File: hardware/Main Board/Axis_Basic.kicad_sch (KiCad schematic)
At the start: 57 parts, among them J1 USB_C_Receptacle_USB2.0, J2 JST_PH, J3 JST_PH, J4 S2B-PH-K-S, J5 1175-1628-ND, J6 1-84952-4, SW1 RKB2SJK, SW2 RKB2SJK, U1 TLV493D, U2 UA78M33CDCYR, U3 ATSAMD51J19A-AUT, U4 TMC2209-LA, U5 AT25040B-MAHL-T, Y1 SG-210STF 48.0000ML0

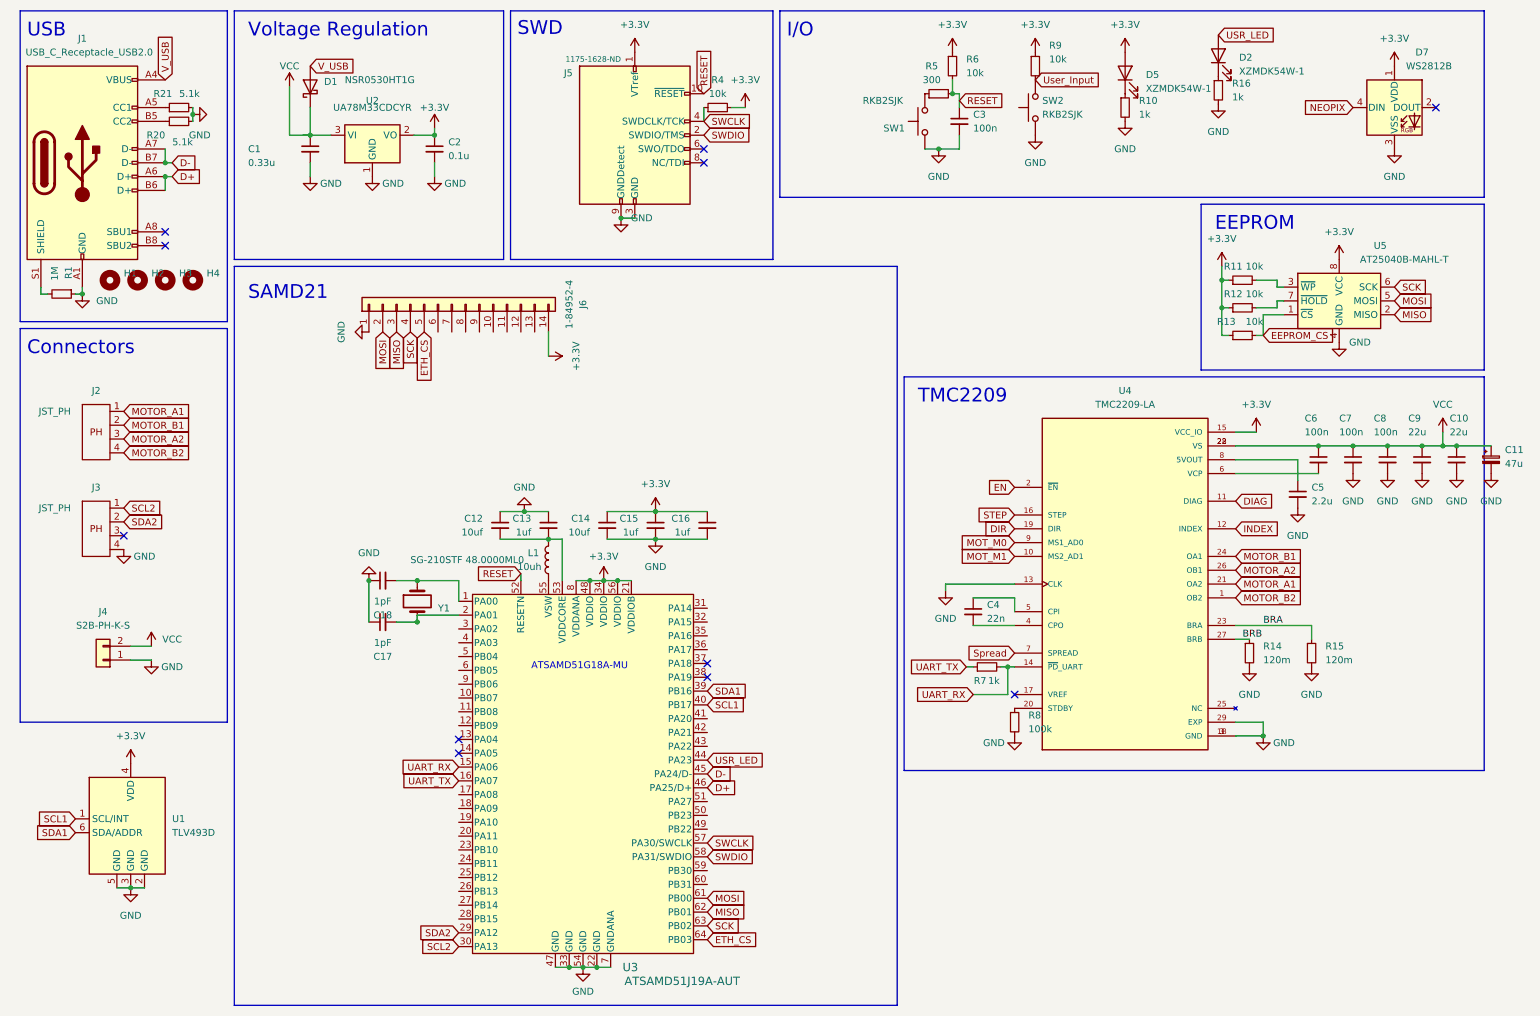
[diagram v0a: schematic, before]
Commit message: PCB V2 draft
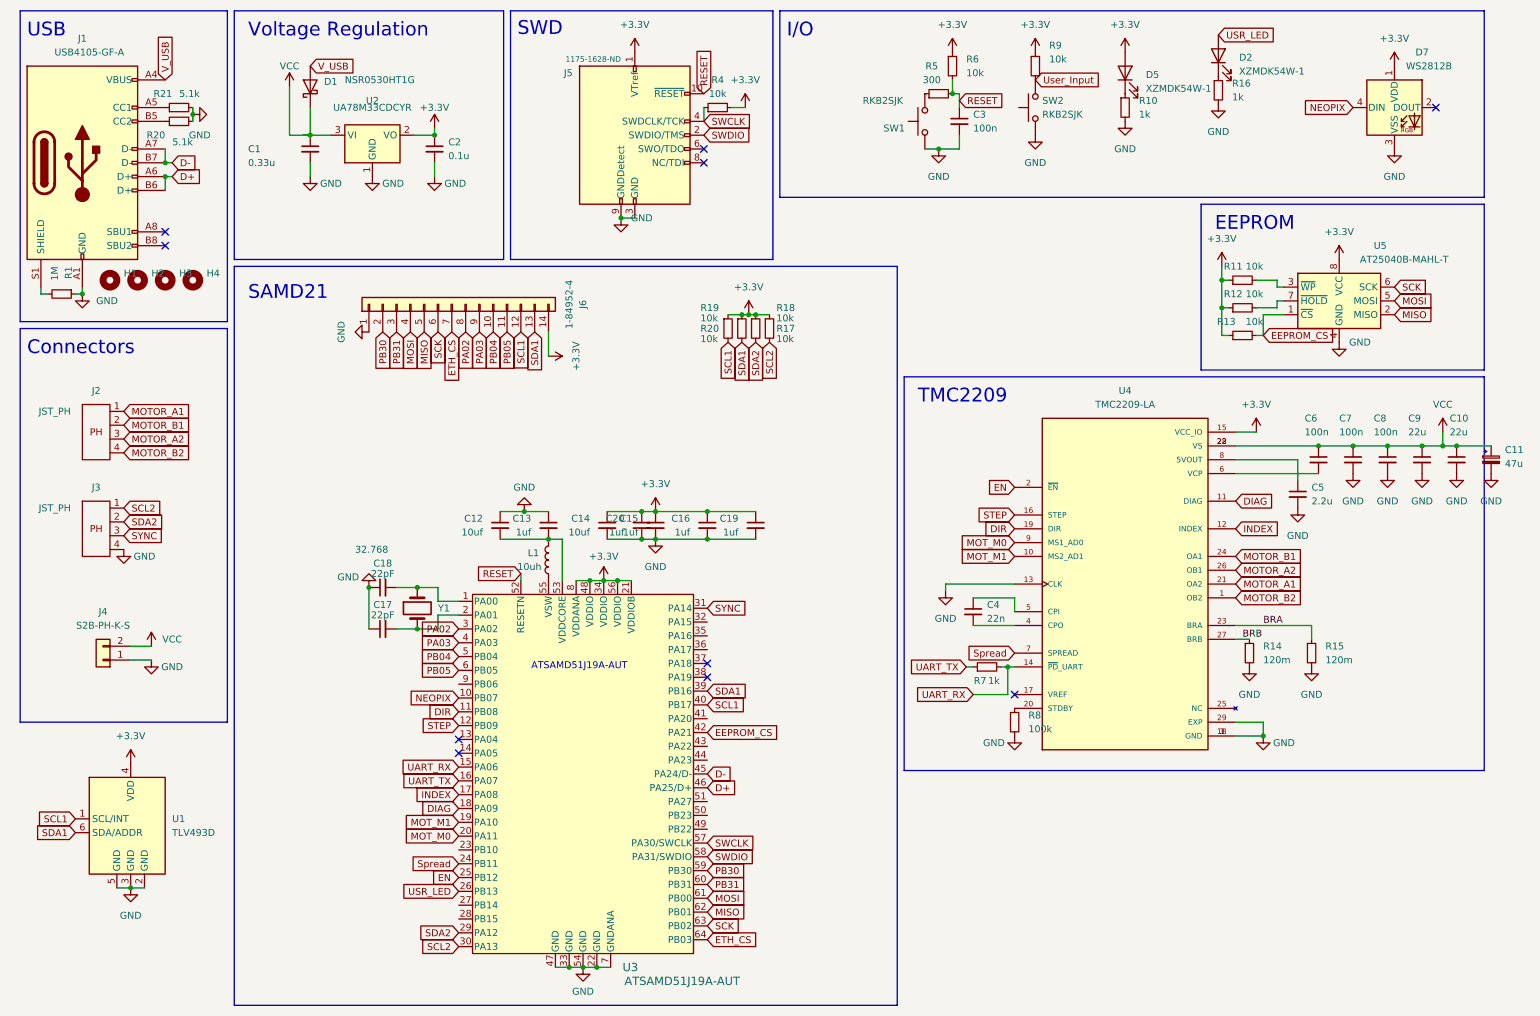
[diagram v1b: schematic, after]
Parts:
- added C19, C20: 1uf, Capacitor_SMD:C_0402_1005Metric, symbol Device:C_Small
- added R17, R18, R19, R20: 10k, Resistor_SMD:R_0402_1005Metric, symbol Device:R_Small
- C17, C18: value 1pF -> 22pF
- J1: value USB_C_Receptacle_USB2.0 -> USB4105-GF-A; footprint Connector_USB:USB_C_Receptacle_G-Switch_GT-USB-7010ASV -> Connector_USB:USB_C_Receptacle_GCT_USB4105-xx-A_16P_TopMnt_Horizontal
- Y1: value SG-210STF 48.0000ML0 -> 32.768; footprint Crystal:Crystal_SMD_2520-4Pin_2.5x2.0mm -> Crystal:Crystal_SMD_3215-2Pin_3.2x1.5mm
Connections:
- net +3.3V: now also C19.1, C20.1, R17.1, R18.1, R19.1, R20.1
- net DIAG: now also U3.18 (PA09)
- net DIR: now also U3.11 (PB08)
- net EEPROM_CS: now also U3.42 (PA21)
- net EN: now also U3.25 (PB12)
- net ETH_CS: now also J6.7 (Pin_7); no longer J6.5 (Pin_5)
- net GND: now also C19.2, C20.2
- net INDEX: now also U3.17 (PA08)
- net MISO: now also J6.5 (Pin_5); no longer J6.3 (Pin_3)
- net MOSI: now also J6.4 (Pin_4); no longer J6.2 (Pin_2)
- net MOT_M0: now also U3.20 (PA11)
- net MOT_M1: now also U3.19 (PA10)
- net NEOPIX: now also U3.10 (PB07)
- net SCK: now also J6.6 (Pin_6); no longer J6.4 (Pin_4)
- net SCL1: now also J6.12 (Pin_12), R20.2
- net SCL2: now also R17.2
- net SDA1: now also J6.13 (Pin_13), R19.2
- net SDA2: now also R18.2
- net STEP: now also U3.12 (PB09)
- net Spread: now also U3.24 (PB11)
- net USR_LED: now also U3.26 (PB13); no longer U3.44 (PA23)
- net PB04: now reaches J6.10 (Pin_10)
- net PB04: now also U3.5 (PB04)
- net PB05: now reaches J6.11 (Pin_11)
- net PB05: now also U3.6 (PB05)
- net PA02: now reaches J6.8 (Pin_8)
- net PA02: now also U3.3 (PA02)
- net PA03: now reaches J6.9 (Pin_9)
- net PA03: now also U3.4 (PA03)
- net SYNC: now reaches U3.31 (PA14)
- net SYNC: now also J3.3
- net PB30: now reaches U3.59 (PB30)
- net PB30: now also J6.2 (Pin_2)
- net PB31: now reaches U3.60 (PB31)
- net PB31: now also J6.3 (Pin_3)
- no-connect marks 11 -> 10
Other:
- note added: "ATSAMD51J19A-AUT"
- note removed: "ATSAMD51G18A-MU"
- moved on the sheet: C17, C18, Y1
